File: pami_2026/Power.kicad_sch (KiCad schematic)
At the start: 13 parts, among them J1 Conn_01x02_Pin, Q1 PMOS, U2 AZ1117CH2-3.3, U3 AZ1117CH2-3.3, U4 TB67H420FTG_O_EL_

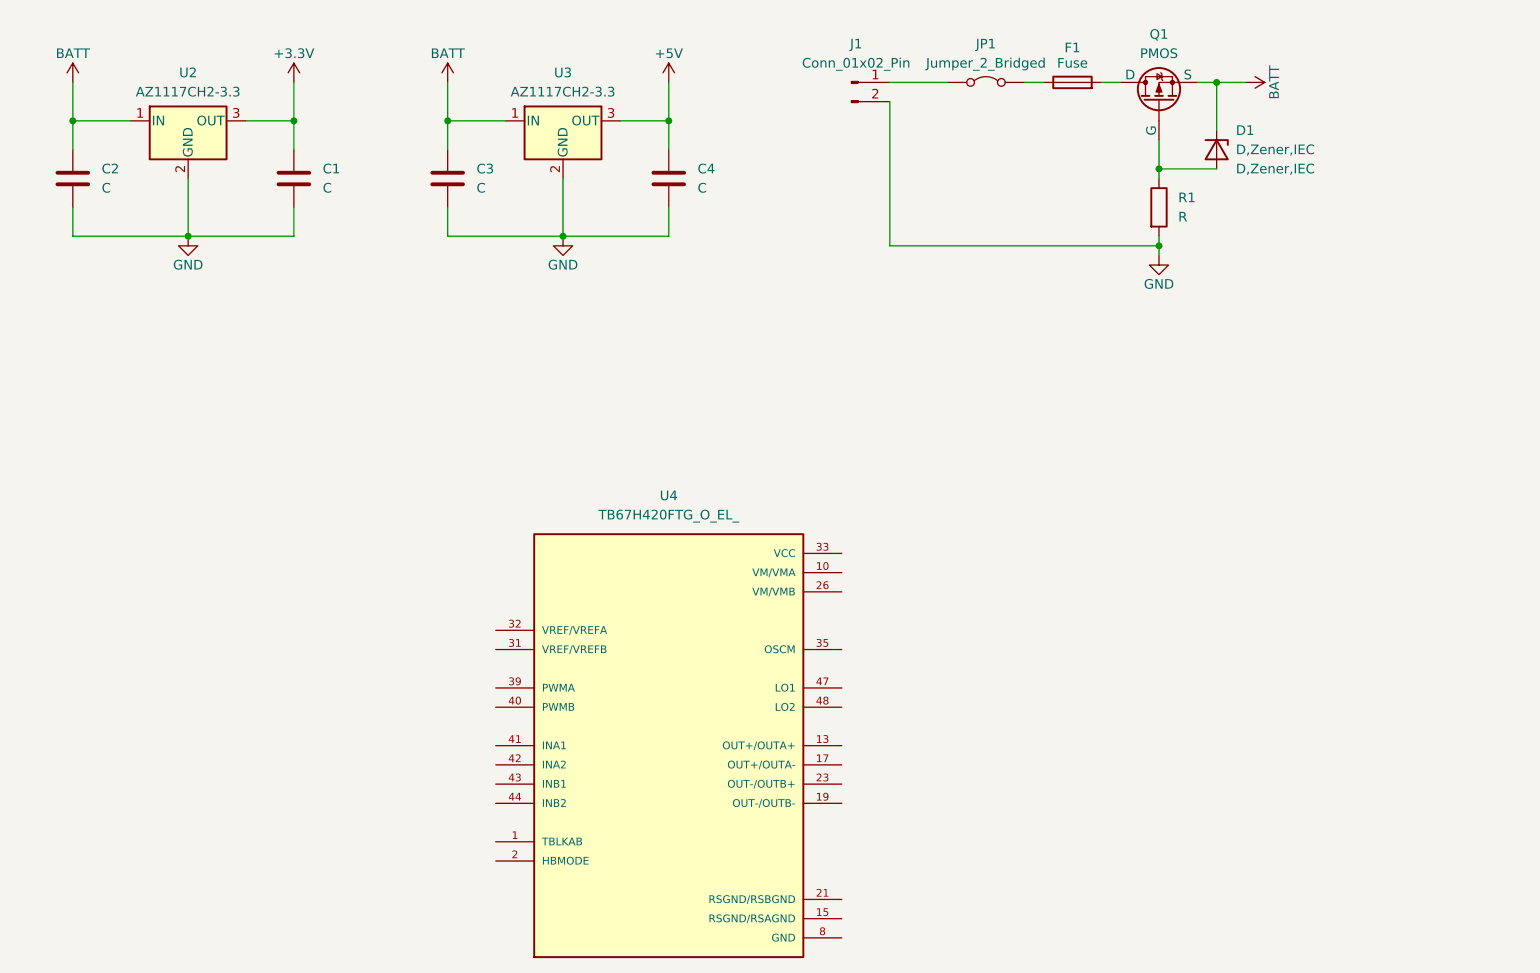
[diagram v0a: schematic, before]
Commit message: WIP alim stage
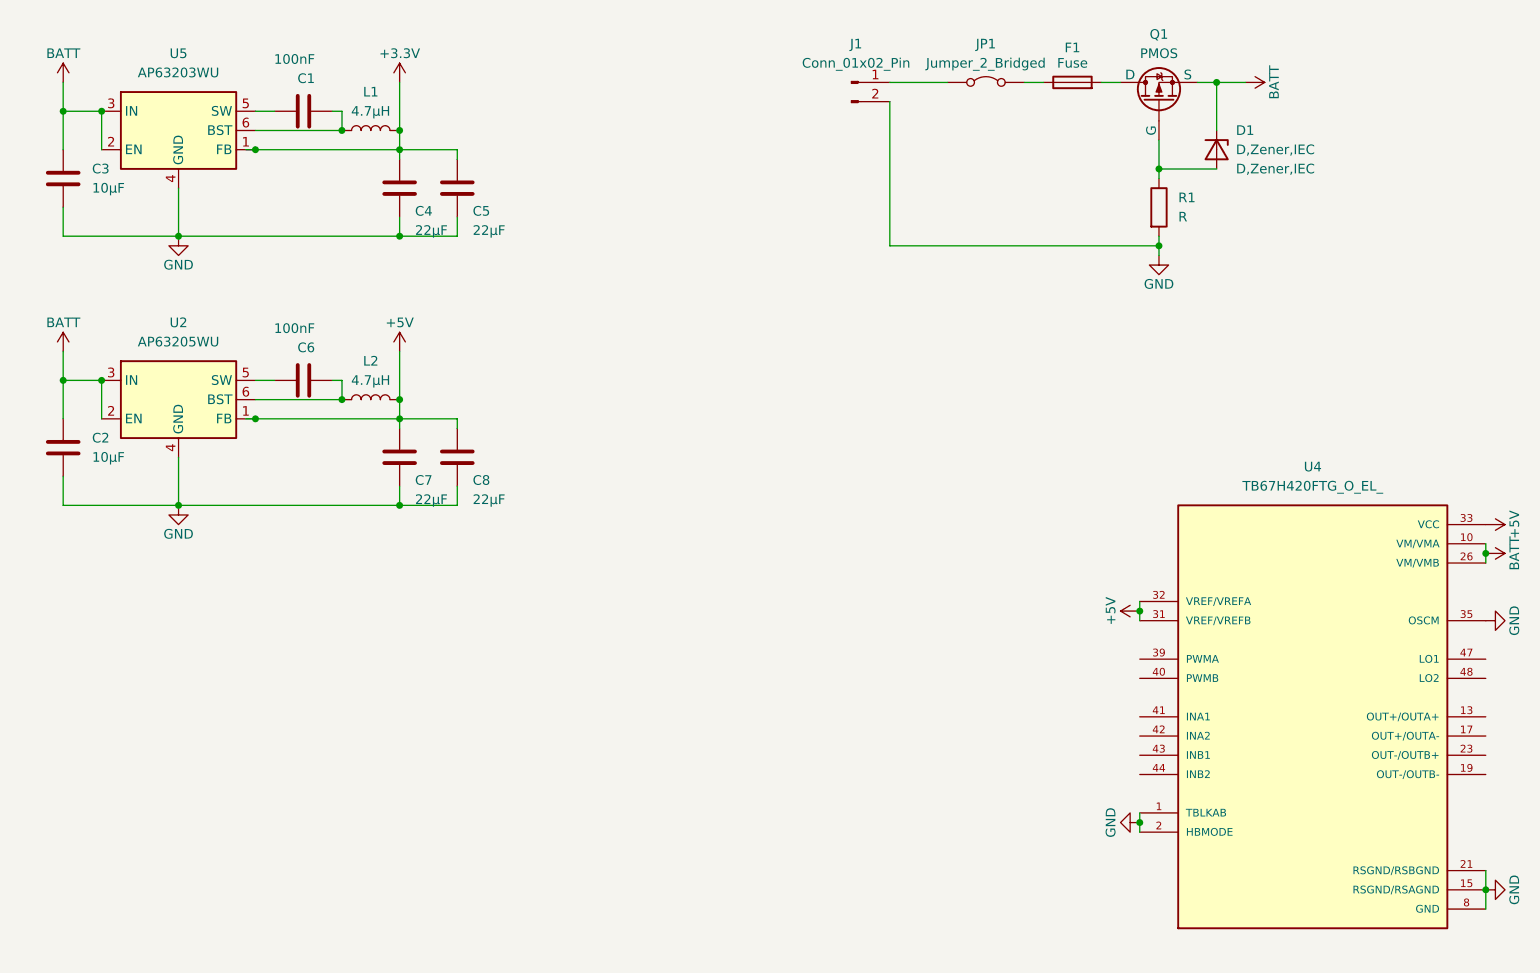
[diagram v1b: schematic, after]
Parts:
- removed U2, U3: AZ1117CH2-3.3, Package_TO_SOT_SMD:SOT-223-3_TabPin2, symbol Regulator_Linear:AZ1117CH2-3.3
- added C5, C7, C8: 22µF, Capacitor_SMD:C_0201_0603Metric, symbol Device:C
- added C6: 100nF, Capacitor_SMD:C_0201_0603Metric, symbol Device:C
- added L1, L2: 4.7µH, Inductor_SMD_Wurth:L_Wurth_WE-LQSH-4020, symbol Device:L
- added U2: AP63205WU, Package_TO_SOT_SMD:TSOT-23-6, symbol Regulator_Switching:AP63205WU
- added U5: AP63203WU, Package_TO_SOT_SMD:TSOT-23-6, symbol Regulator_Switching:AP63203WU
- C1: value C -> 100nF; footprint (none) -> Capacitor_SMD:C_0201_0603Metric
- C2, C3: value C -> 10µF; footprint (none) -> Capacitor_SMD:C_0201_0603Metric
- C4: value C -> 22µF; footprint (none) -> Capacitor_SMD:C_0201_0603Metric
- R1: footprint (none) -> Resistor_SMD:R_0201_0603Metric
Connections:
- net RSGND/RSAGND is gone; now on net GND: U4.15 (RSGND/RSAGND), U4.16 (RSGND/RSAGND)
- net RSGND/RSBGND is gone; now on net GND: U4.21 (RSGND/RSBGND), U4.22 (RSGND/RSBGND)
- net VCC is gone; now on net +5V: U4.33 (VCC), U4.34 (VCC)
- net VM/VMA is gone; now on net BATT: U4.10 (VM/VMA), U4.11 (VM/VMA)
- net VM/VMB is gone; now on net BATT: U4.26 (VM/VMB), U4.27 (VM/VMB)
- net +3.3V: now also C4.1, C5.1, L1.2, U5.1 (FB); no longer C1.1
- net +5V: now also U4.31 (VREF/VREFB), U4.32 (VREF/VREFA), C7.1, C8.1, L2.2, U2.1 (FB); no longer C4.1
- net BATT: now also U2.2 (EN), U2.3 (IN), U5.2 (EN), U5.3 (IN)
- net GND: now also U4.1 (TBLKAB), U4.2 (HBMODE), U4.35 (OSCM), C5.2, C7.2, C8.2, U2.4 (GND), U5.4 (GND); no longer C1.2
- new net: C6.2, L2.1, U2.6 (BST)
- new net: C6.1, U2.5 (SW)
- new net: C1.1, U5.5 (SW)
- new net: C1.2, L1.1, U5.6 (BST)
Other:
- moved on the sheet: C3, C4, U4

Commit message: WIP actuators
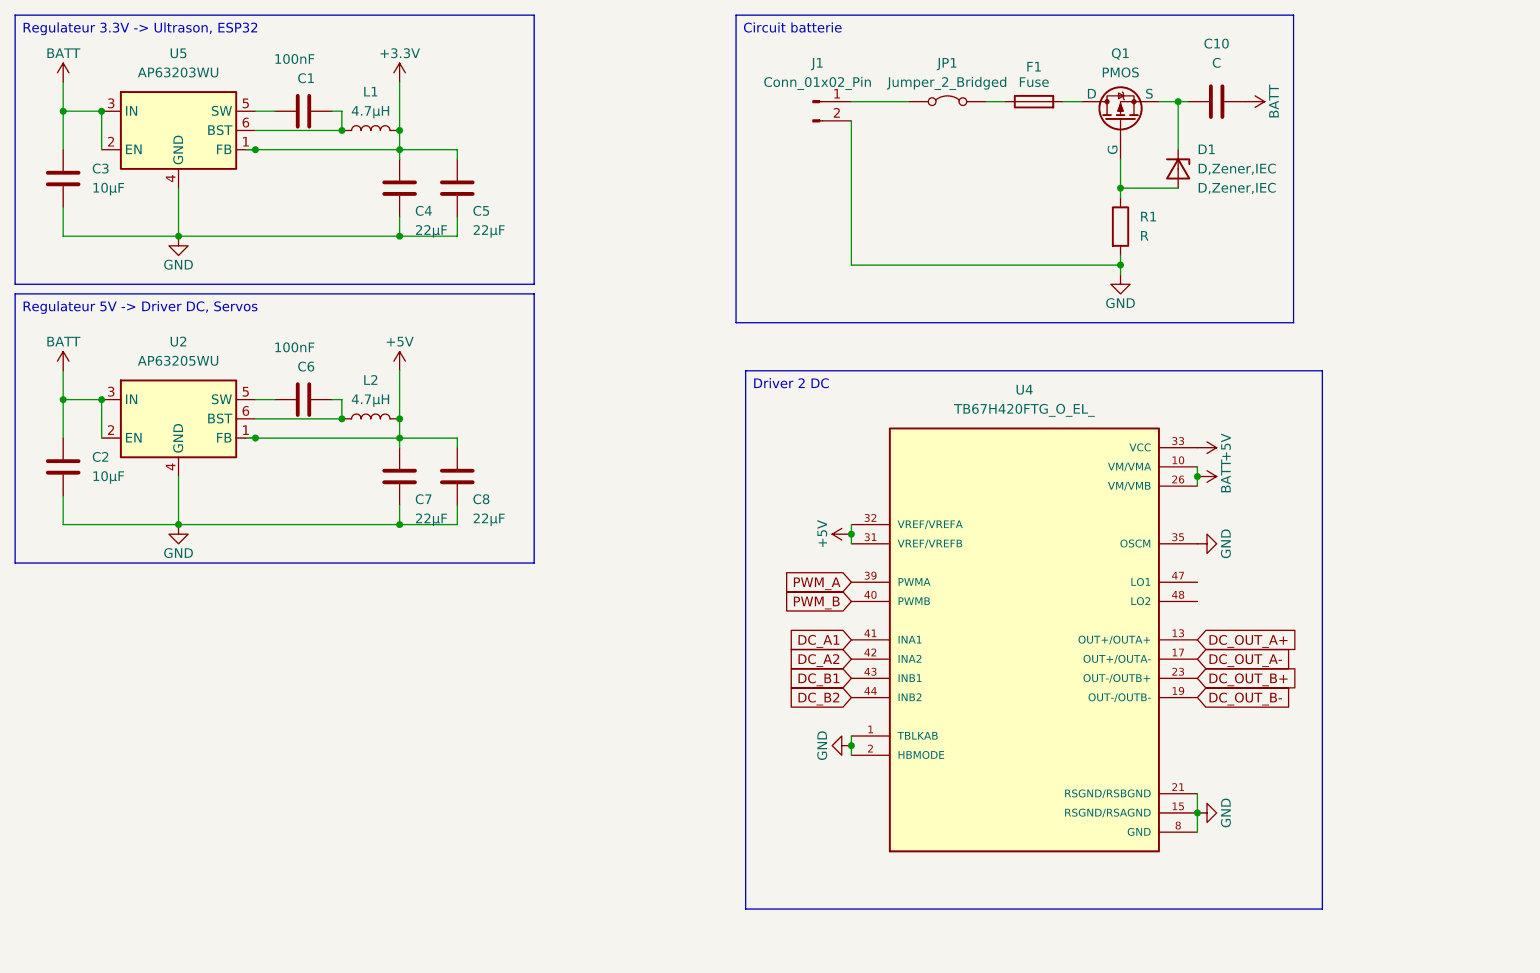
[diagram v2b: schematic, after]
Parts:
- added C10: C, symbol Device:C
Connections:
- net BATT: now also C10.2; no longer D1.1 (K-), Q1.3 (S)
- net DC_OUT_A+: now reaches U4.13 (OUT+/OUTA+), U4.14 (OUT+/OUTA+)
- net DC_OUT_A-: now reaches U4.17 (OUT+/OUTA-), U4.18 (OUT+/OUTA-)
- net DC_OUT_B-: now reaches U4.19 (OUT-/OUTB-), U4.20 (OUT-/OUTB-)
- net DC_OUT_B+: now reaches U4.23 (OUT-/OUTB+), U4.24 (OUT-/OUTB+)
- net PWM_A: now reaches U4.39 (PWMA)
- net PWM_B: now reaches U4.40 (PWMB)
- net DC_A1: now reaches U4.41 (INA1)
- net DC_A2: now reaches U4.42 (INA2)
- net DC_B1: now reaches U4.43 (INB1)
- net DC_B2: now reaches U4.44 (INB2)
- new net: C10.1, D1.1 (K-), Q1.3 (S)
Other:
- moved on the sheet: C2, C6, C7, C8, D1, F1, J1, JP1, L2, Q1, R1, U2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
